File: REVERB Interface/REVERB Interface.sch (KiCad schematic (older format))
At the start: 23 parts, among them J1 RPiZeroW, J10 USB, J2 Iridium, J3 APRS, J4 Antenna, J5 MAX3232BOB, J6 USBSER2, J7 USBSER3, J8 USBSER1, J9 USB, M1 MountingHole_Pad, M2 MountingHole_Pad, M3 MountingHole_Pad, M4 MountingHole_Pad, U2 MAX3232, U3 SC16IS752IPW

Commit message: do stuff
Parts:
- removed U3: SC16IS752IPW, Package_SO:TSSOP-28_4.4x9.7mm_P0.65mm, symbol Interface_UART:SC16IS752IPW
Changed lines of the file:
@@
-$EndComp
-$Comp
-L Interface_UART:SC16IS752IPW U3
-U 1 1 615DC7E1
-P 10950 2750
-F 0 "U3" H 10950 3931 50  0000 C CNN
-F 1 "SC16IS752IPW" H 10950 3840 50  0000 C CNN
-F 2 "Package_SO:TSSOP-28_4.4x9.7mm_P0.65mm" H 10950 1200 50  0001 C CNN
-F 3 "https://www.nxp.com/docs/en/data-sheet/SC16IS752_SC16IS762.pdf" H 10950 1350 50  0001 C CNN
-	1    10950 2750
-	1    0    0    -1
 $EndComp
 $Comp

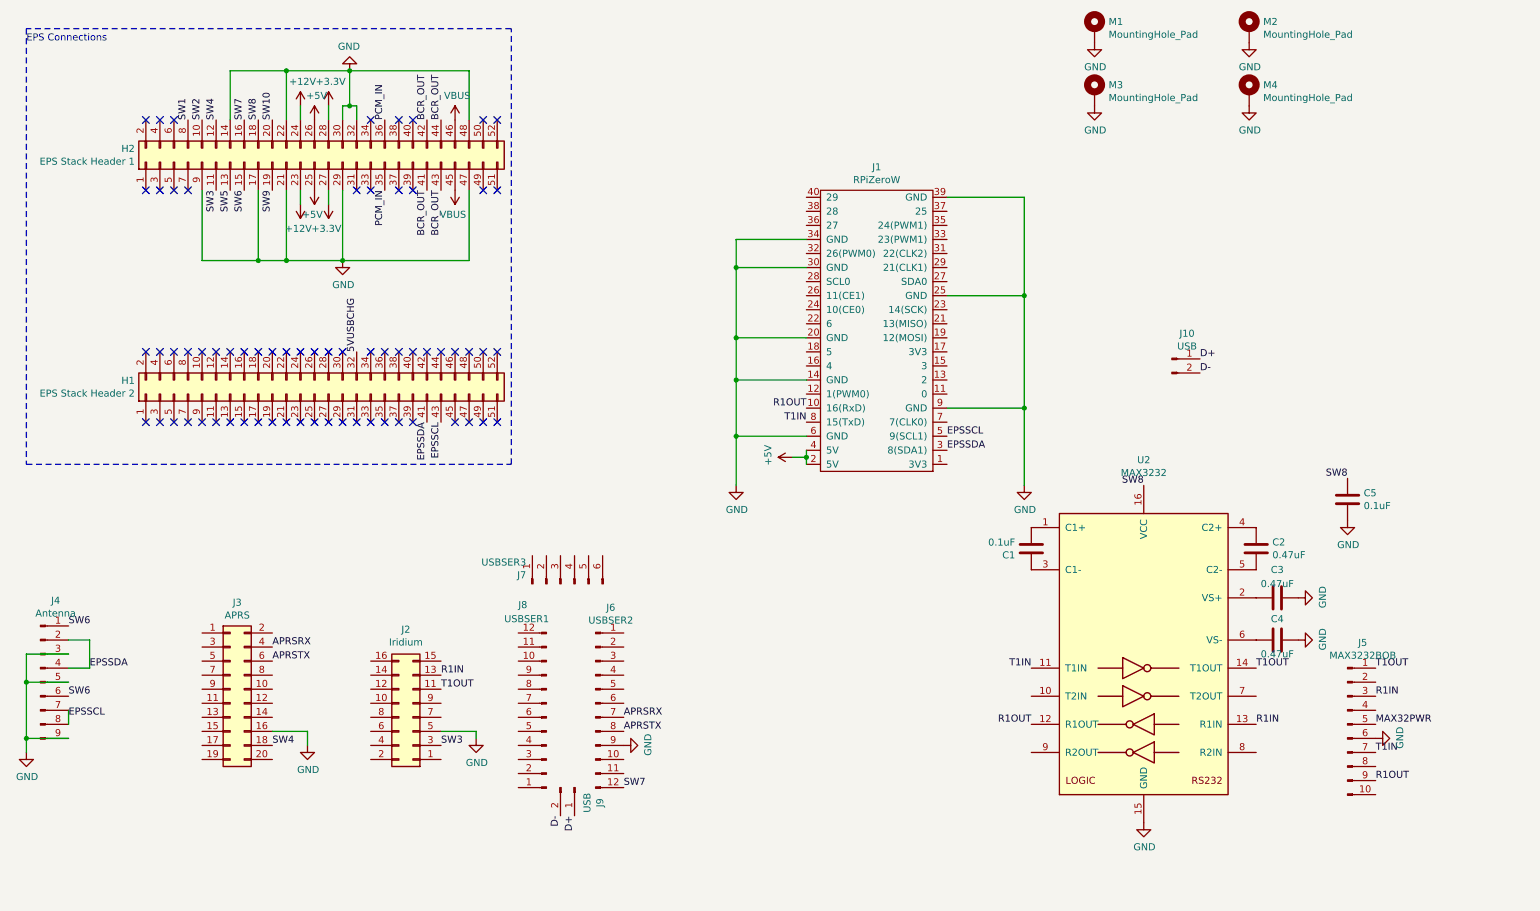
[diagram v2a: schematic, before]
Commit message: bunch of work
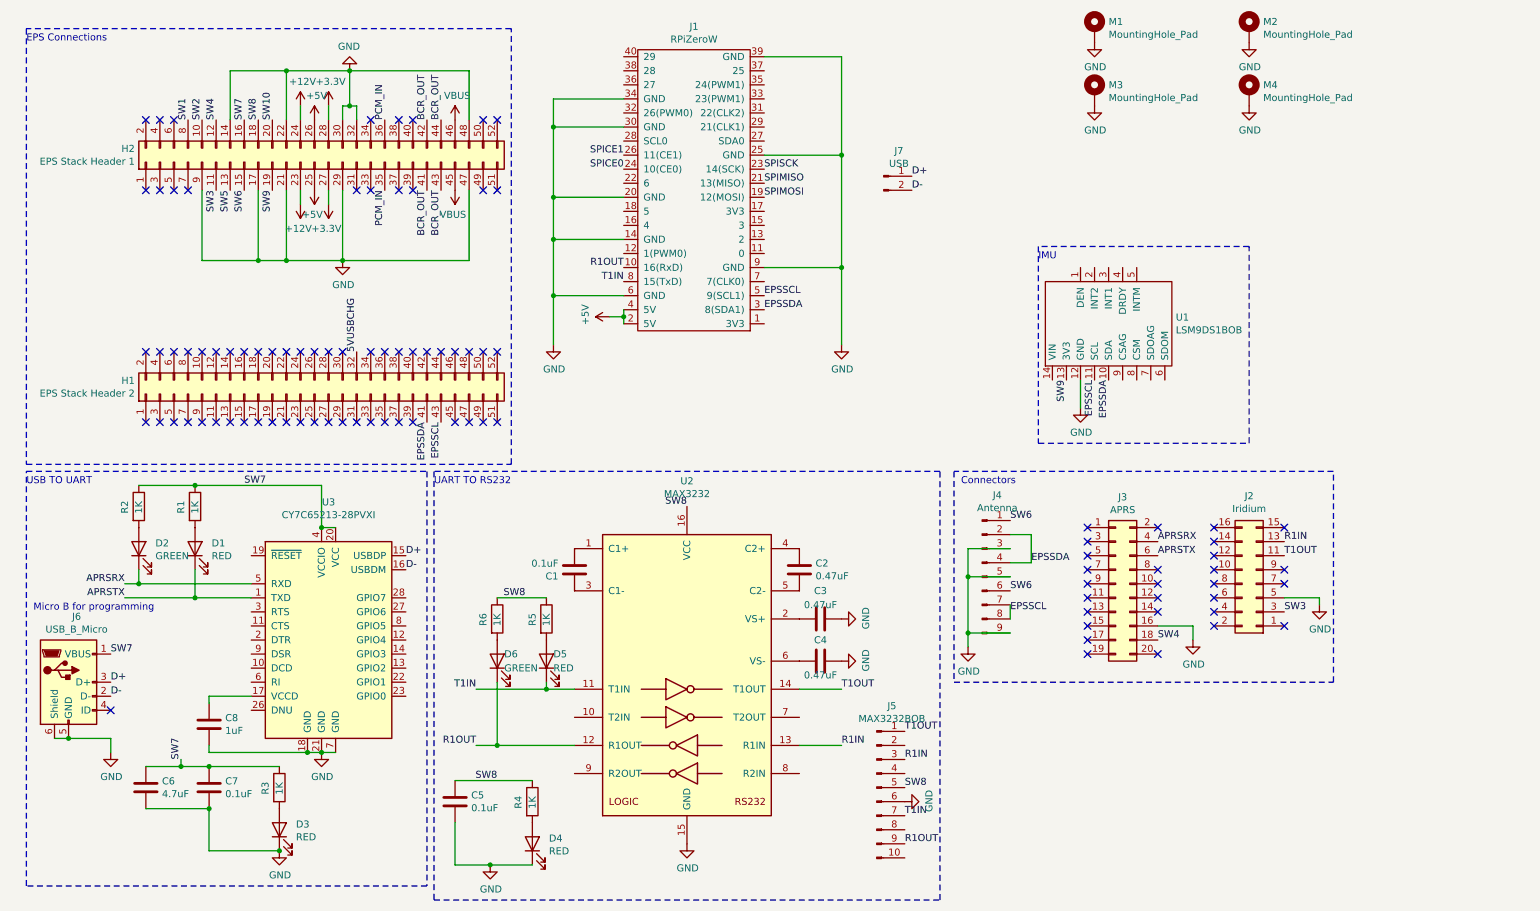
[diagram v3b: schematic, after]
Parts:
- removed J6: USBSER2, Connector_PinSocket_2.54mm:PinSocket_1x12_P2.54mm_Vertical, symbol Connector:Conn_01x12_Male
- removed J7: USBSER3, Connector_PinSocket_2.54mm:PinSocket_1x06_P2.54mm_Vertical, symbol Connector:Conn_01x06_Male
- removed J8: USBSER1, Connector_PinSocket_2.54mm:PinSocket_1x12_P2.54mm_Vertical, symbol Connector:Conn_01x12_Male
- removed J9: USB, Connector_PinSocket_2.54mm:PinSocket_1x02_P2.54mm_Vertical, symbol Connector:Conn_01x02_Male
- added C6: 4.7uF, Capacitor_SMD:C_0805_2012Metric_Pad1.18x1.45mm_HandSolder, symbol Device:C
- added C7: 0.1uF, Capacitor_SMD:C_0805_2012Metric_Pad1.18x1.45mm_HandSolder, symbol Device:C
- added C8: 1uF, Capacitor_SMD:C_0805_2012Metric_Pad1.18x1.45mm_HandSolder, symbol Device:C
- added D1, D3, D4, D5: RED, LED_SMD:LED_0805_2012Metric_Pad1.15x1.40mm_HandSolder, symbol Device:LED
- added D2, D6: GREEN, LED_SMD:LED_0805_2012Metric_Pad1.15x1.40mm_HandSolder, symbol Device:LED
- added J6: USB_B_Micro, REVERB Interface:AdafruitMicroB, symbol Connector:USB_B_Micro
- added R1, R2, R3, R4, R5, R6: 1K, Resistor_SMD:R_1206_3216Metric_Pad1.30x1.75mm_HandSolder, symbol Device:R
- added U1: LSM9DS1BOB, REVERB Interface:LSM9DS1BOB, symbol REVERBSym:LSM9DS1BOB
- added U3: CY7C65213-28PVXI, Package_SO:SSOP-28_5.3x10.2mm_P0.65mm, symbol Interface_USB:CY7C65213-28PVXI
- renumbered J10 to J7
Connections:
- net MAX32PWR is gone; now on net SW8: J5.5 (Pin_5)
- net APRSRX: now also D2.1 (K), U3.5 (RXD)
- net APRSTX: now also D1.1 (K), U3.1 (TXD)
- net D+: now also J6.3 (D+), U3.15 (USBDP)
- net D-: now also J6.2 (D-), U3.16 (USBDM)
- net EPSSCL: now also U1.11 (SCL)
- net EPSSDA: now also U1.10 (SDA)
- net GND: now also C6.2, C7.2, C8.2, D3.1 (K), D4.1 (K), J6.5 (GND), J6.6 (Shield), U1.12 (GND), U3.18 (GND), U3.21 (GND), U3.7 (GND)
- net R1OUT: now also D6.1 (K)
- net SW7: now also C6.1, C7.1, J6.1 (VBUS), R1.1, R2.1, R3.1, U3.20 (VCC), U3.4 (VCCIO)
- net SW8: now also R4.1, R5.1, R6.1
- net SW9: now also U1.13 (3V3)
- net T1IN: now also D5.1 (K)
- net SPIMOSI: now reaches J1.19 (12(MOSI))
- net SPIMISO: now reaches J1.21 (13(MISO))
- net SPISCK: now reaches J1.23 (14(SCK))
- net SPICE0: now reaches J1.24 (10(CE0))
- net SPICE1: now reaches J1.26 (11(CE1))
- new net: C8.1, U3.17 (VCCD)
- new net: D1.2 (A), R1.2
- new net: D2.2 (A), R2.2
- new net: D3.2 (A), R3.2
- new net: D4.2 (A), R4.2
- new net: D5.2 (A), R5.2
- new net: D6.2 (A), R6.2
- no-connect marks 67 -> 96
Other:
- note added: "Connectors"
- note added: "IMU"
- note added: "Micro B for programming"
- note added: "UART TO RS232"
- note added: "USB TO UART"
- moved on the sheet: C1, C2, C3, C4, C5, J1, J2, J3, J4, J5, J7, U2
